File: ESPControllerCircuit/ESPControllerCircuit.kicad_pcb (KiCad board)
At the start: 2 copper layers, 5 parts, among them J1 Conn_01x02_Female, SW1 SW_Push, U1 WeMos_mini

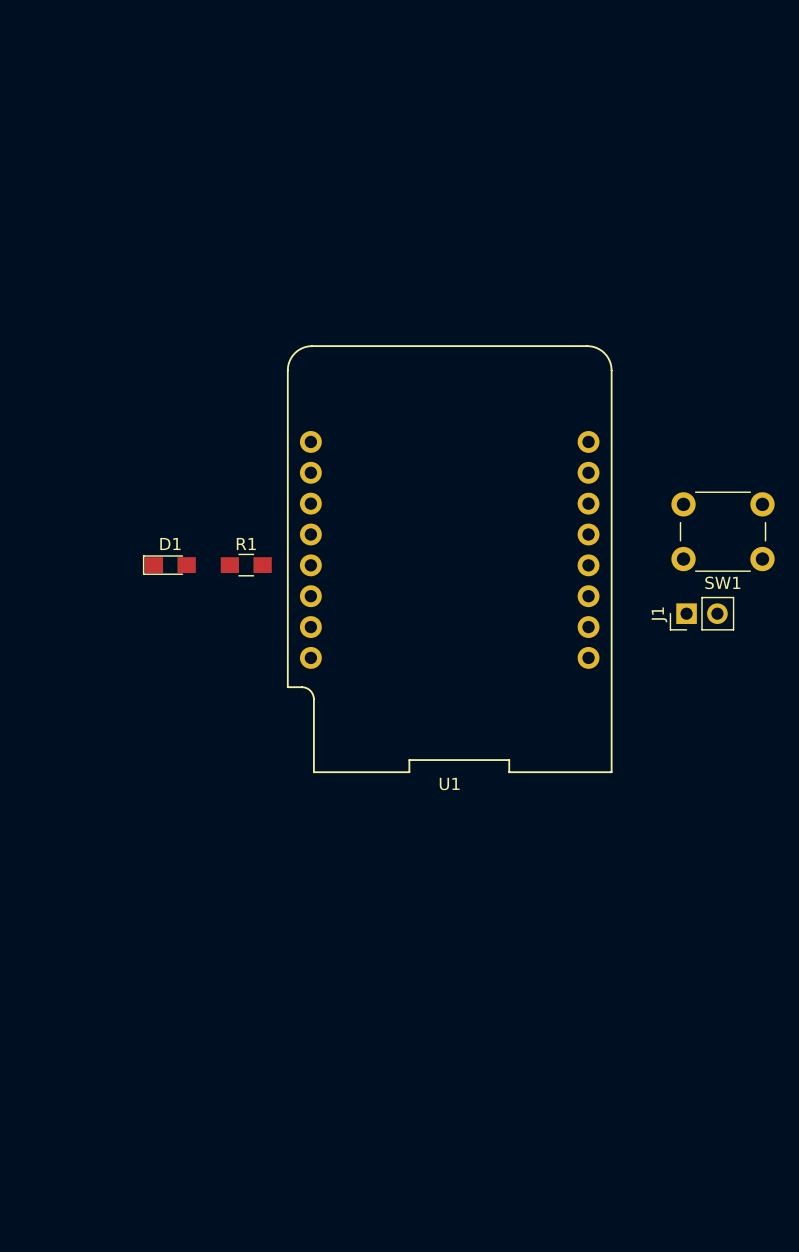
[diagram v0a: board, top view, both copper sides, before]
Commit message: Basic controller circuit
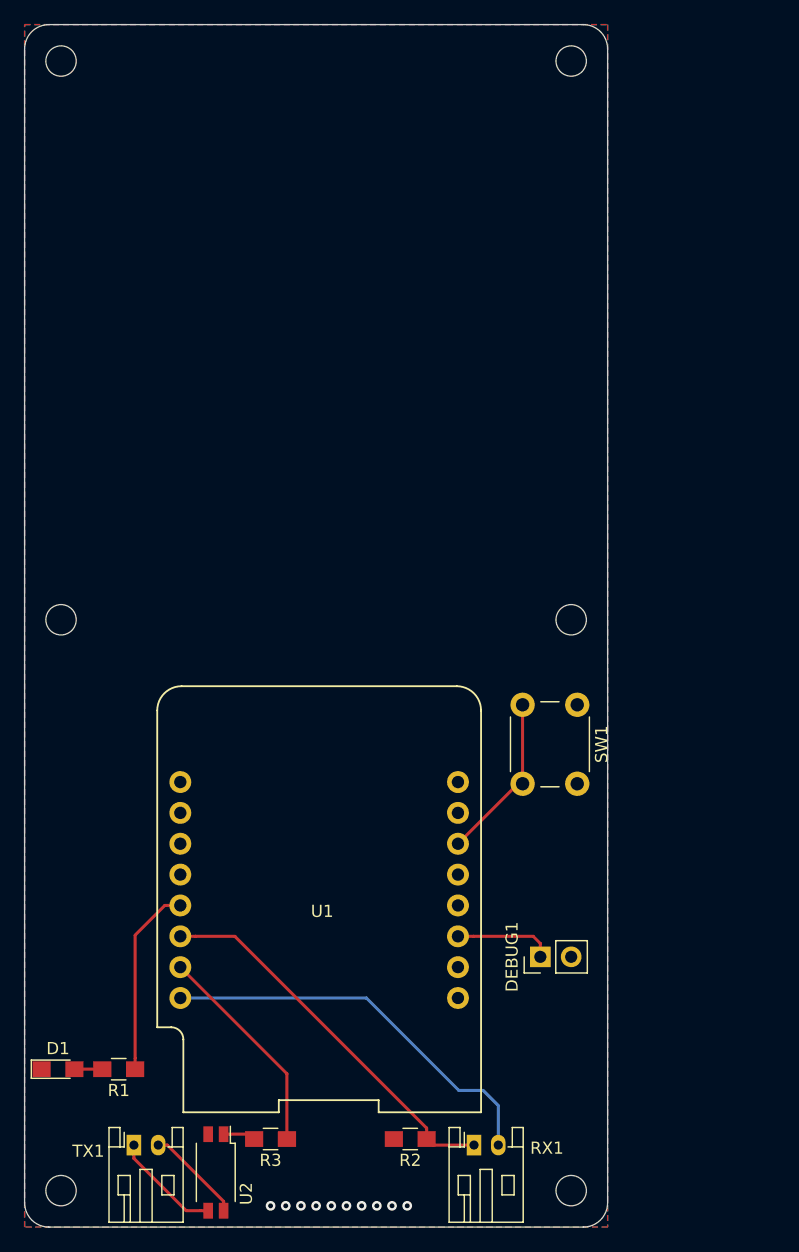
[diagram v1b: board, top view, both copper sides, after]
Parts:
- removed J1: Conn_01x02_Female, Pin_Headers:Pin_Header_Straight_1x02_Pitch2.54mm
- added DEBUG1: Conn_01x02_Female, Pin_Headers:Pin_Header_Straight_1x02_Pitch2.54mm, F.Cu at (142.5, 137.8)
- added R2: 470R, Resistors_SMD:R_0805_HandSoldering, F.Cu at (131.8, 152.8)
- added R3: 220R, Resistors_SMD:R_0805_HandSoldering, F.Cu at (120.2, 152.8)
- added REF**: MountingHole_2.5mm, Mounting_Holes:MountingHole_2.5mm, F.Cu at (103.0, 110.0)
- added REF**: MountingHole_2.5mm, Mounting_Holes:MountingHole_2.5mm, F.Cu at (145.0, 110.0)
- added REF**: MountingHole_2.5mm, Mounting_Holes:MountingHole_2.5mm, F.Cu at (145.0, 64.0)
- added REF**: MountingHole_2.5mm, Mounting_Holes:MountingHole_2.5mm, F.Cu at (103.0, 64.0)
- added REF**: MountingHole_2.5mm, Mounting_Holes:MountingHole_2.5mm, F.Cu at (103.0, 157.0)
- added REF**: MountingHole_2.5mm, Mounting_Holes:MountingHole_2.5mm, F.Cu at (145.0, 157.0)
- added RX1: Conn_01x02_Male, Connectors_JST:JST_PH_S2B-PH-K_02x2.00mm_Angled, F.Cu at (137.0, 153.2)
- added TX1: Conn_01x02_Male, Connectors_JST:JST_PH_S2B-PH-K_02x2.00mm_Angled, F.Cu at (109.0, 153.2)
- added U2: HMHA2801, Housings_SSOP:SOP-4_4.4x2.8mm_Pitch1.27mm, F.Cu at (115.8, 155.5)
- D1: value LED -> COMMS
- R1: value 512R -> 470R
- moved R1 42.8 mm to (107.8, 147.0)
- moved D1 42.5 mm to (102.8, 147.0)
- moved U1 30.0 mm to (124.2, 132.2)
- moved SW1 19.4 mm to (145.5, 117.0), turned to 270 degrees
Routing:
- net +3V3: track 0.00 -> 33.1 mm
- net Net-(R2-Pad2): track 0.00 -> 31.8 mm
- net Net-(R3-Pad2): track 0.00 -> 17.8 mm
- net Net-(R1-Pad2): track 0.00 -> 15.8 mm
- net Net-(SW1-Pad2): track 0.00 -> 13.9 mm
- net Net-(TX1-Pad1): track 0.00 -> 8.99 mm
- net Net-(DEBUG1-Pad1): track 0.00 -> 8.12 mm
- net Net-(TX1-Pad2): track 0.00 -> 8.07 mm
- net Net-(R3-Pad1): track 0.00 -> 2.68 mm
- net Net-(D1-Pad2): track 0.00 -> 2.30 mm
- net GND: vias 0 -> 10
- added copper zone on B.Cu, net GND
- added copper zone on F.Cu, net GND
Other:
- board outline added: 48 x 99 mm
